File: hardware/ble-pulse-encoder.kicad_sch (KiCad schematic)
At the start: 55 parts, among them J1 USB_B_Micro, J2 EZmate-3, J3 EZmate-4, J4 TC2030-IDC-NL, J5 EZmate-5, Q1 BSS84, Q2 Q_Photo_NPN_CBE, Q3 Q_Photo_NPN_CBE, SW1 SW_Push, U1 STBC08, U2 nRF52832-QFxx, U3 TPS7A0333DBVR, Y1 32.768kHz, Y2 32MHz

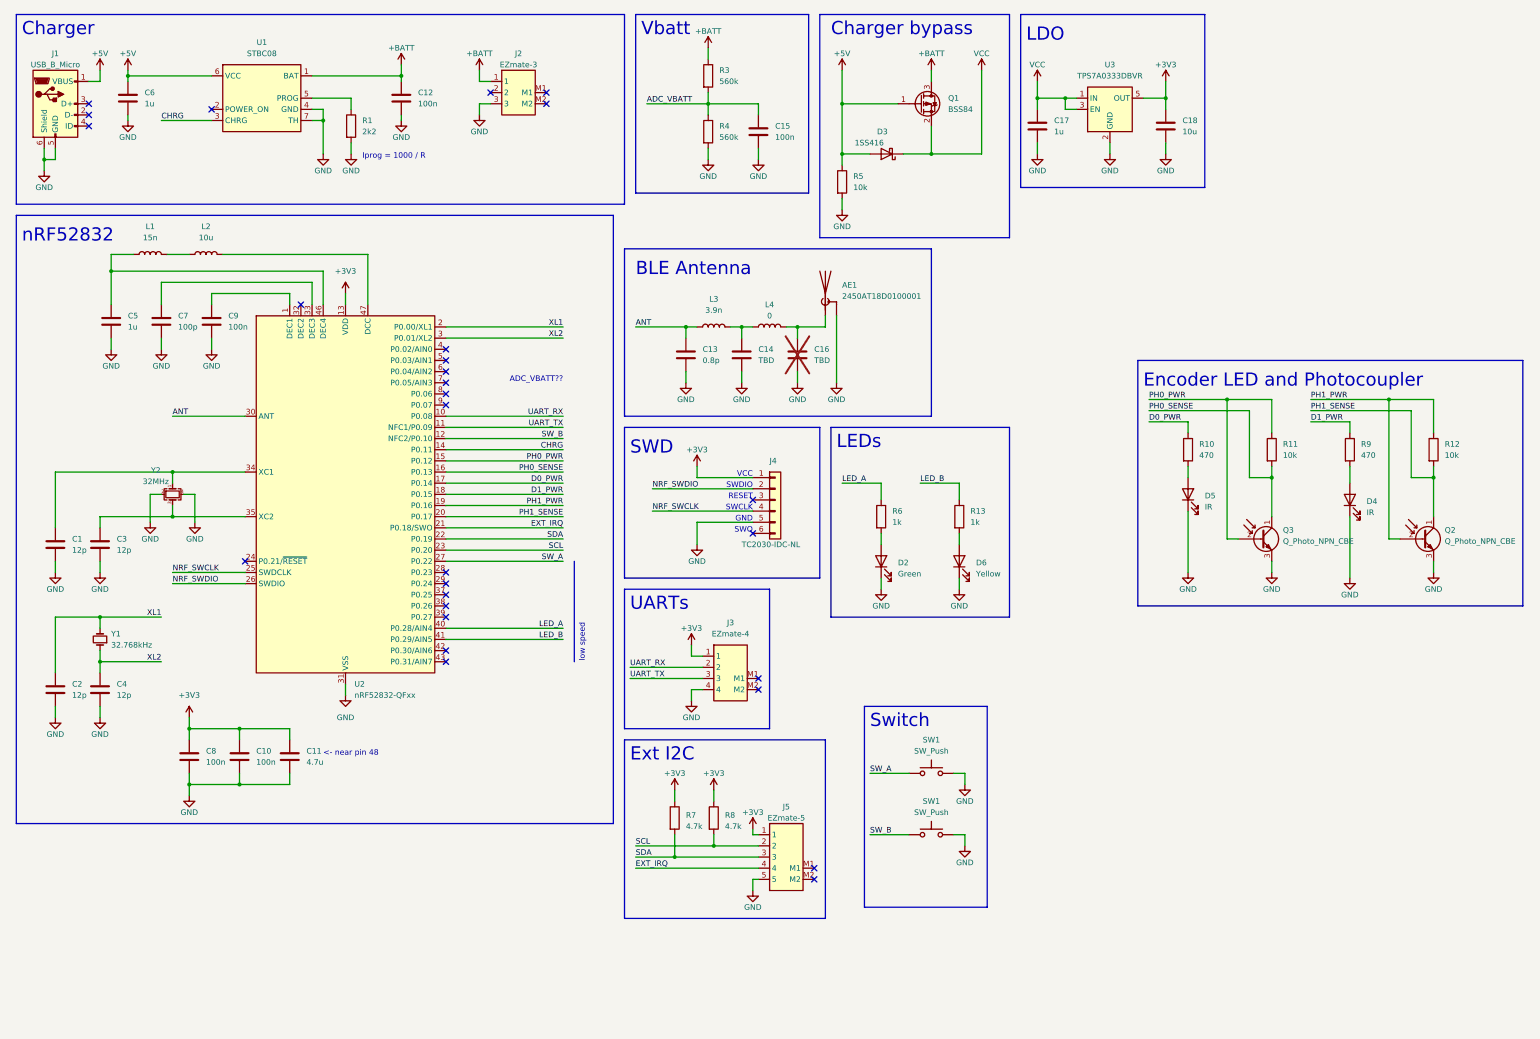
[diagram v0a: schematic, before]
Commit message: hw: r1
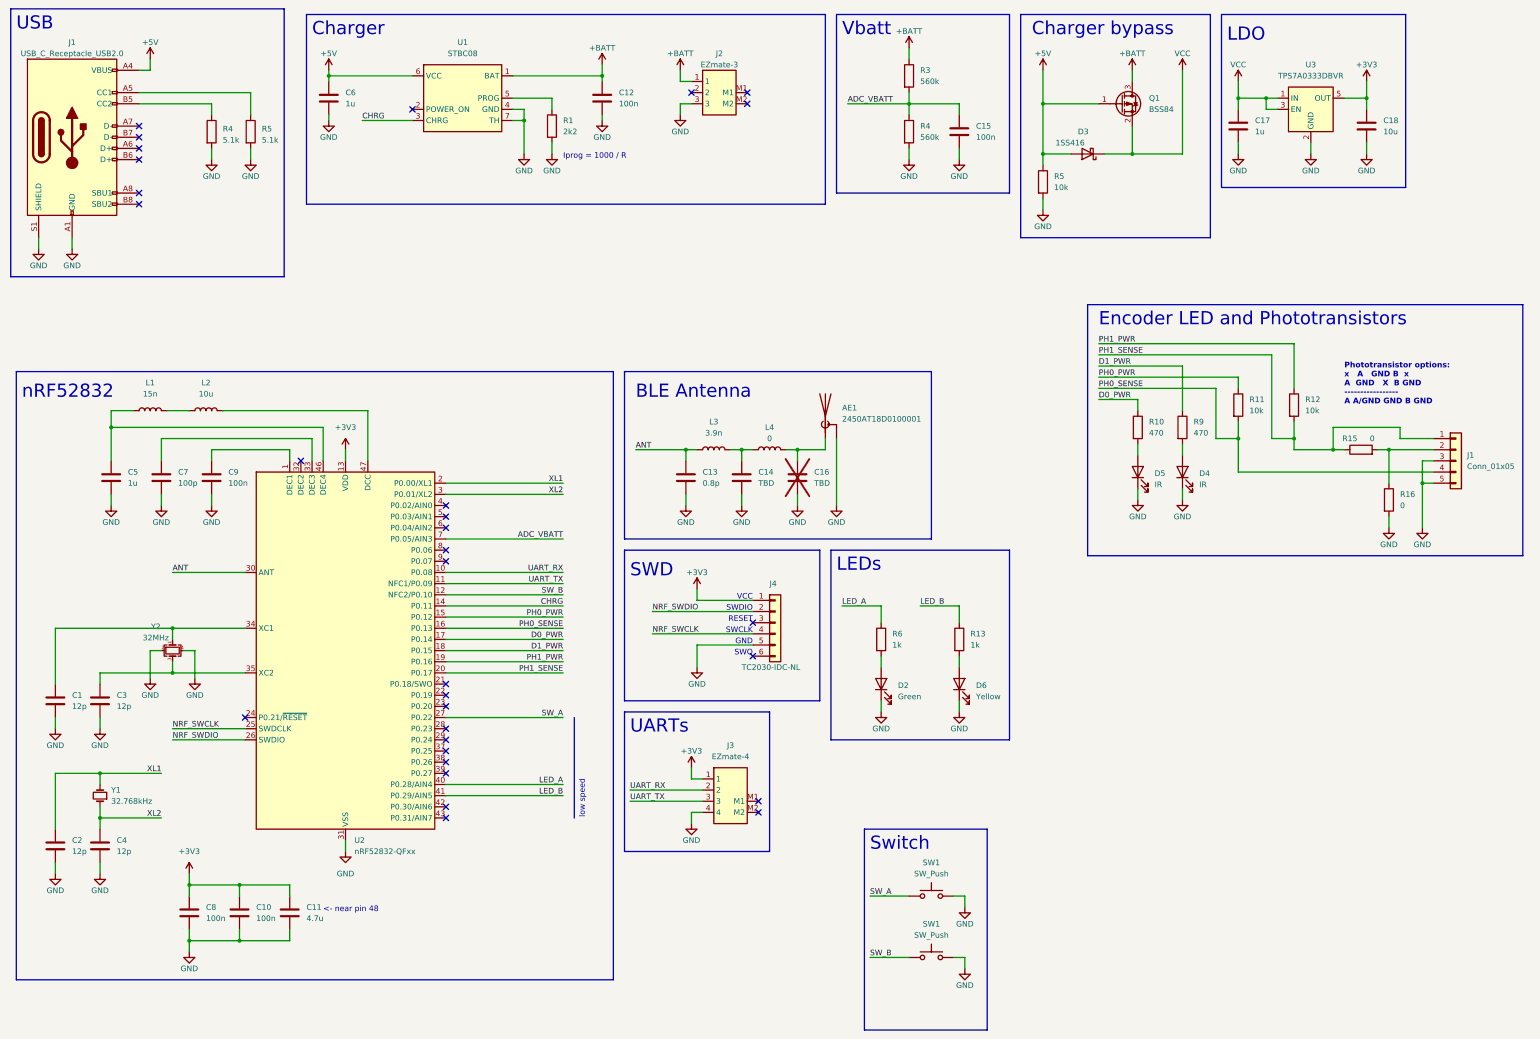
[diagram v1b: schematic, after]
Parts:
- removed J1: USB_B_Micro, Connector_USB:USB_Micro-B_Amphenol_10104110_Horizontal, symbol Connector:USB_B_Micro
- removed J5: EZmate-5, balto:EZmate-5, symbol balto:EZmate-5
- removed Q2, Q3: Q_Photo_NPN_CBE, Connector_PinHeader_2.00mm:PinHeader_1x03_P2.00mm_Vertical, symbol Device:Q_Photo_NPN_CBE
- removed R7, R8: 4.7k, balto:R_0402_Worthington, symbol Device:R
- added J1: Conn_01x05, Connector_PinHeader_2.00mm:PinHeader_1x05_P2.00mm_Vertical, symbol Connector_Generic:Conn_01x05
- added J1: USB_C_Receptacle_USB2.0, Connector_USB:USB_C_Receptacle_JAE_DX07S016JA1R1500, symbol Connector:USB_C_Receptacle_USB2.0
- added R15, R16: 0, balto:R_0402_Worthington, symbol Device:R
- added R4, R5: 5.1k, balto:R_0402_Worthington, symbol Device:R
- AE1: footprint balto:2450AT18D0100001-R -> balto:2450AT18D0100001-L
- R11, R12: footprint Resistor_SMD:R_0603_1608Metric -> balto:R_0402_Worthington
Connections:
- net +5V: now also J1.A4 (VBUS), J1.A9 (VBUS), J1.B4 (VBUS), J1.B9 (VBUS)
- net ADC_VBATT: now also U2.7 (P0.05/AIN3)
- net GND: now also J1.3 (Pin_3), J1.5 (Pin_5), J1.A1 (GND), J1.A12 (GND), J1.B1 (GND), J1.B12 (GND), J1.S1 (SHIELD), R16.2, R4.2, R5.2
- net PH0_SENSE: now also J1.4 (Pin_4)
- net PH1_SENSE: now also J1.1 (Pin_1), R15.1
- net EXT_IRQ: no longer names the net of U2.21 (P0.18/SWO)
- net SCL: no longer names the net of U2.23 (P0.20)
- net SDA: no longer names the net of U2.22 (P0.19)
- new net: J1.A5 (CC1), R5.1
- new net: J1.2 (Pin_2), R15.2, R16.1
- new net: J1.B5 (CC2), R4.1
- no-connect marks 28 -> 31
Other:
- note added: "Encoder LED and Phototransistors"
- note added: "Phototransistor options: x A GND B x A GND X B GND ----------------- A A/GND GND B GND"
- note added: "USB"
- note removed: "ADC_VBATT??"
- note removed: "Encoder LED and Photocoupler"
- note removed: "Ext I2C"
- moved on the sheet: AE1, C1, C10, C11, C12, C13, C14, C15, C16, C17, C18, C2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
